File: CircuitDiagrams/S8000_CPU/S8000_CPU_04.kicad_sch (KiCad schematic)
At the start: 8 parts, among them U14 74113, U32 7404, U33 7411, U41 7432, U43 Z80 CTC, U44 Z80 CTC, U81 7414

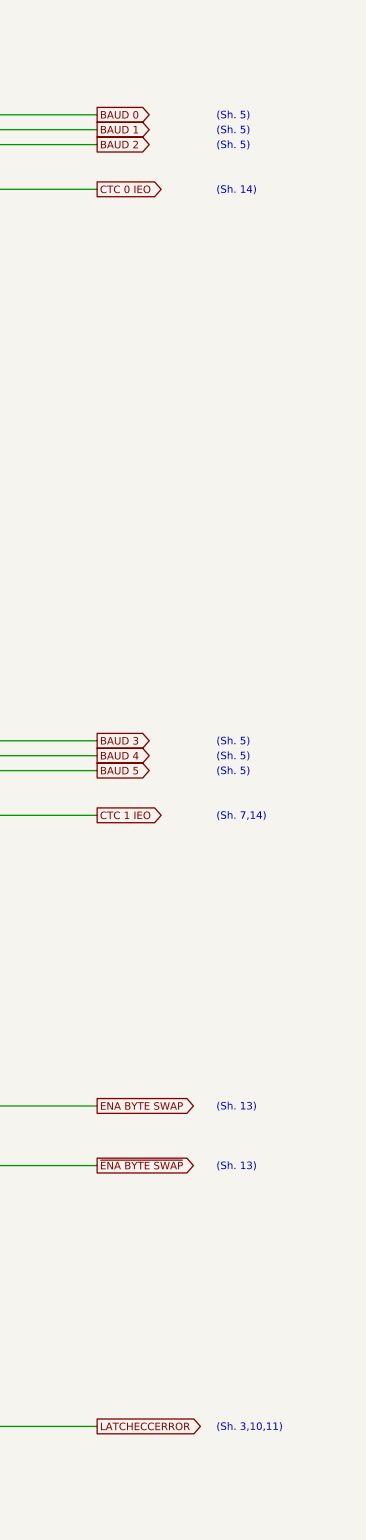
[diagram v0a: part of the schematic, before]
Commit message: Add Page 5 (SIO 0+1)
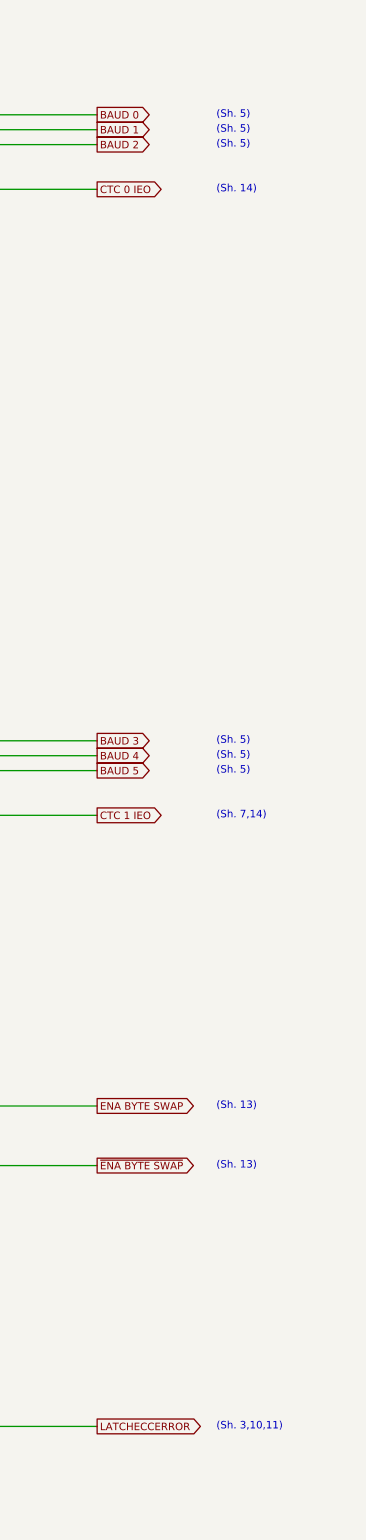
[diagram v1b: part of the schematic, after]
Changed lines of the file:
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@@
 	(text "(Sh. 7,14)"
 		(exclude_from_sim no)
-		(at 553.72 228.854 0)
+		(at 553.72 228.6 0)
 		(effects
 			(font
@@
 	(text "(Sh. 5)"
 		(exclude_from_sim no)
-		(at 553.72 218.694 0)
+		(at 553.72 218.44 0)
 		(effects
 			(font
@@
 	(text "(Sh. 13)"
 		(exclude_from_sim no)
-		(at 553.72 278.384 0)
-		(effects
-			(font
-				(size 1.27 1.27)
-			)
-			(justify left)
-		)
-	)
-	(text "(Sh. 5)"
-		(exclude_from_sim no)
-		(at 553.72 216.154 0)
+		(at 553.72 278.13 0)
+		(effects
+			(font
+				(size 1.27 1.27)
+			)
+			(justify left)
+		)
+	)
+	(text "(Sh. 5)"
+		(exclude_from_sim no)
+		(at 553.72 215.9 0)
 		(effects
 			(font
@@
 	(text "(Sh. 5)"
 		(exclude_from_sim no)
-		(at 553.72 112.014 0)
+		(at 553.72 111.76 0)
 		(effects
 			(font
@@
 	(text "(Sh. 3,10,11)"
 		(exclude_from_sim no)
-		(at 553.72 332.994 0)
+		(at 553.72 332.74 0)
 		(effects
 			(font
@@
 	(text "(Sh. 13)"
 		(exclude_from_sim no)
-		(at 553.72 288.544 0)
-		(effects
-			(font
-				(size 1.27 1.27)
-			)
-			(justify left)
-		)
-	)
-	(text "(Sh. 5)"
-		(exclude_from_sim no)
-		(at 553.72 221.234 0)
+		(at 553.72 288.29 0)
+		(effects
+			(font
+				(size 1.27 1.27)
+			)
+			(justify left)
+		)
+	)
+	(text "(Sh. 5)"
+		(exclude_from_sim no)
+		(at 553.72 220.98 0)
 		(effects
 			(font
@@
 	(text "(Sh. 5)"
 		(exclude_from_sim no)
-		(at 553.72 109.474 0)
+		(at 553.72 109.22 0)
 		(effects
 			(font
@@
 	(text "(Sh. 5)"
 		(exclude_from_sim no)
-		(at 553.72 114.554 0)
+		(at 553.72 114.3 0)
 		(effects
 			(font
@@
 	(text "(Sh. 14)"
 		(exclude_from_sim no)
-		(at 553.72 122.174 0)
-		(effects
-			(font
+		(at 553.72 121.92 0)
+		(effects
+			(font
